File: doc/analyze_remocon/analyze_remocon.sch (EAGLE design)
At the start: 15 parts, among them IC3 PIC18F2550_28DIP, T1 2SC1815, X1 MINI-USB-UX60-MB-5S8

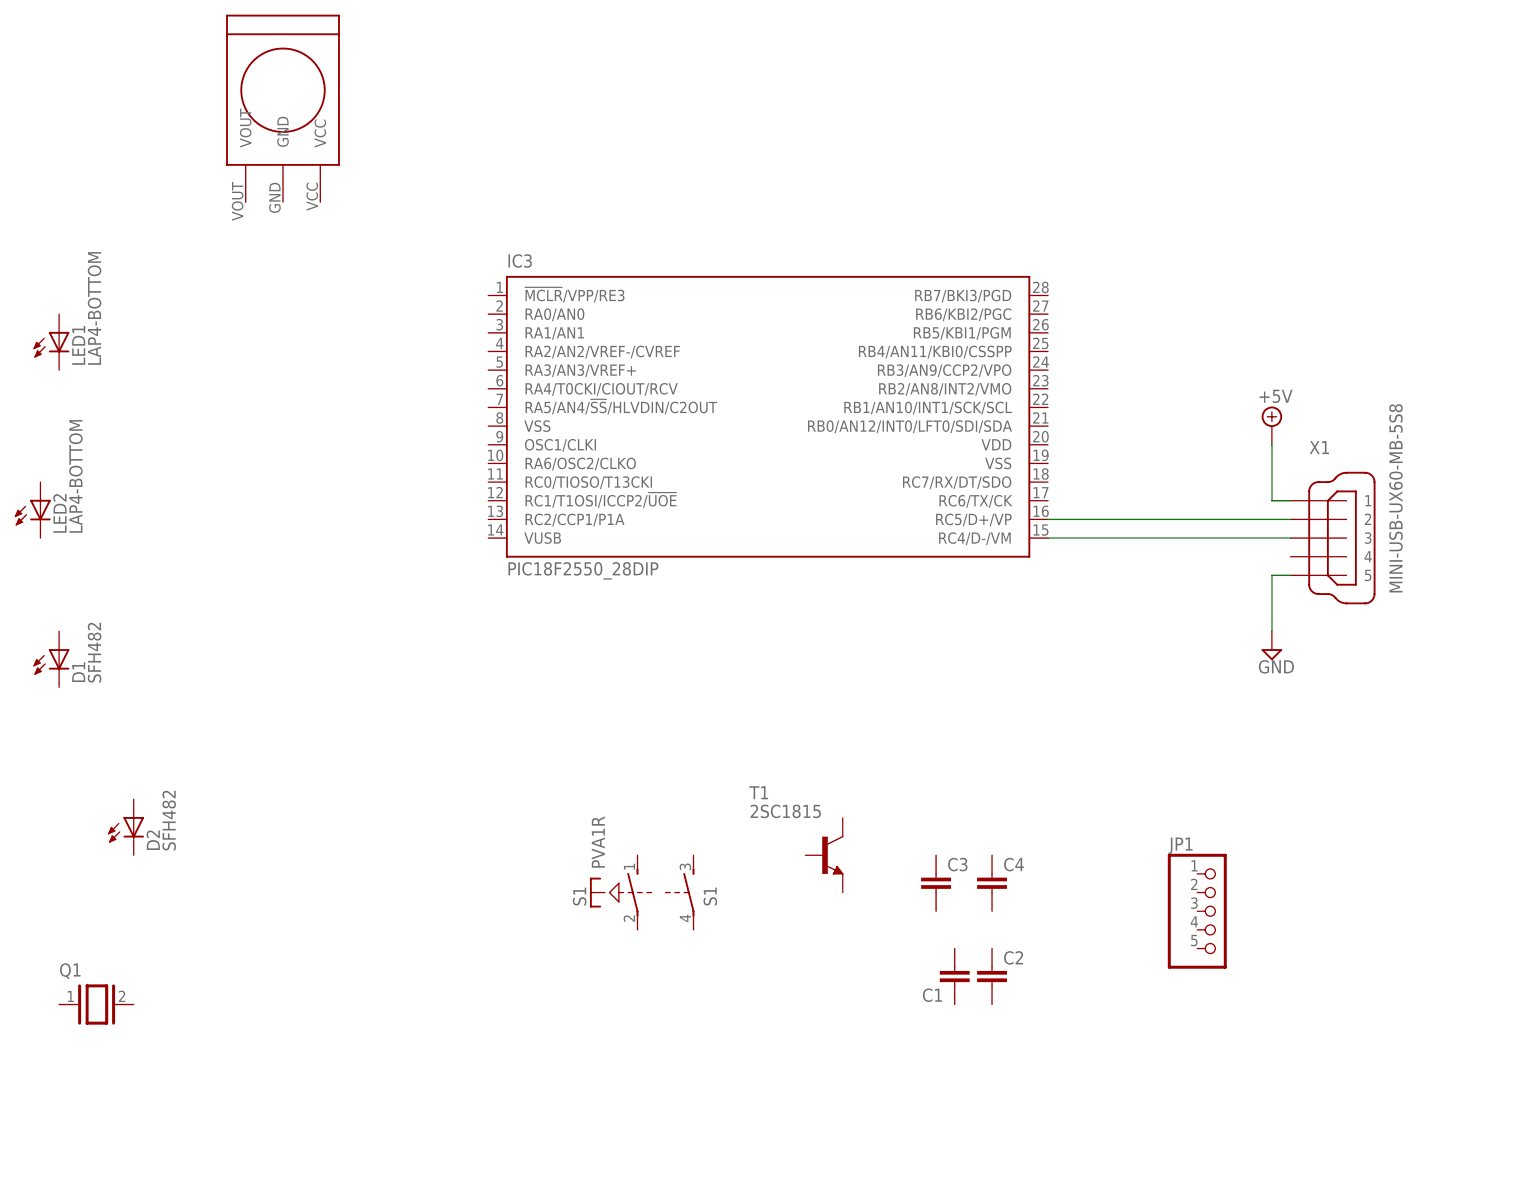
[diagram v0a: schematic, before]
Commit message: update circuit diagram documents
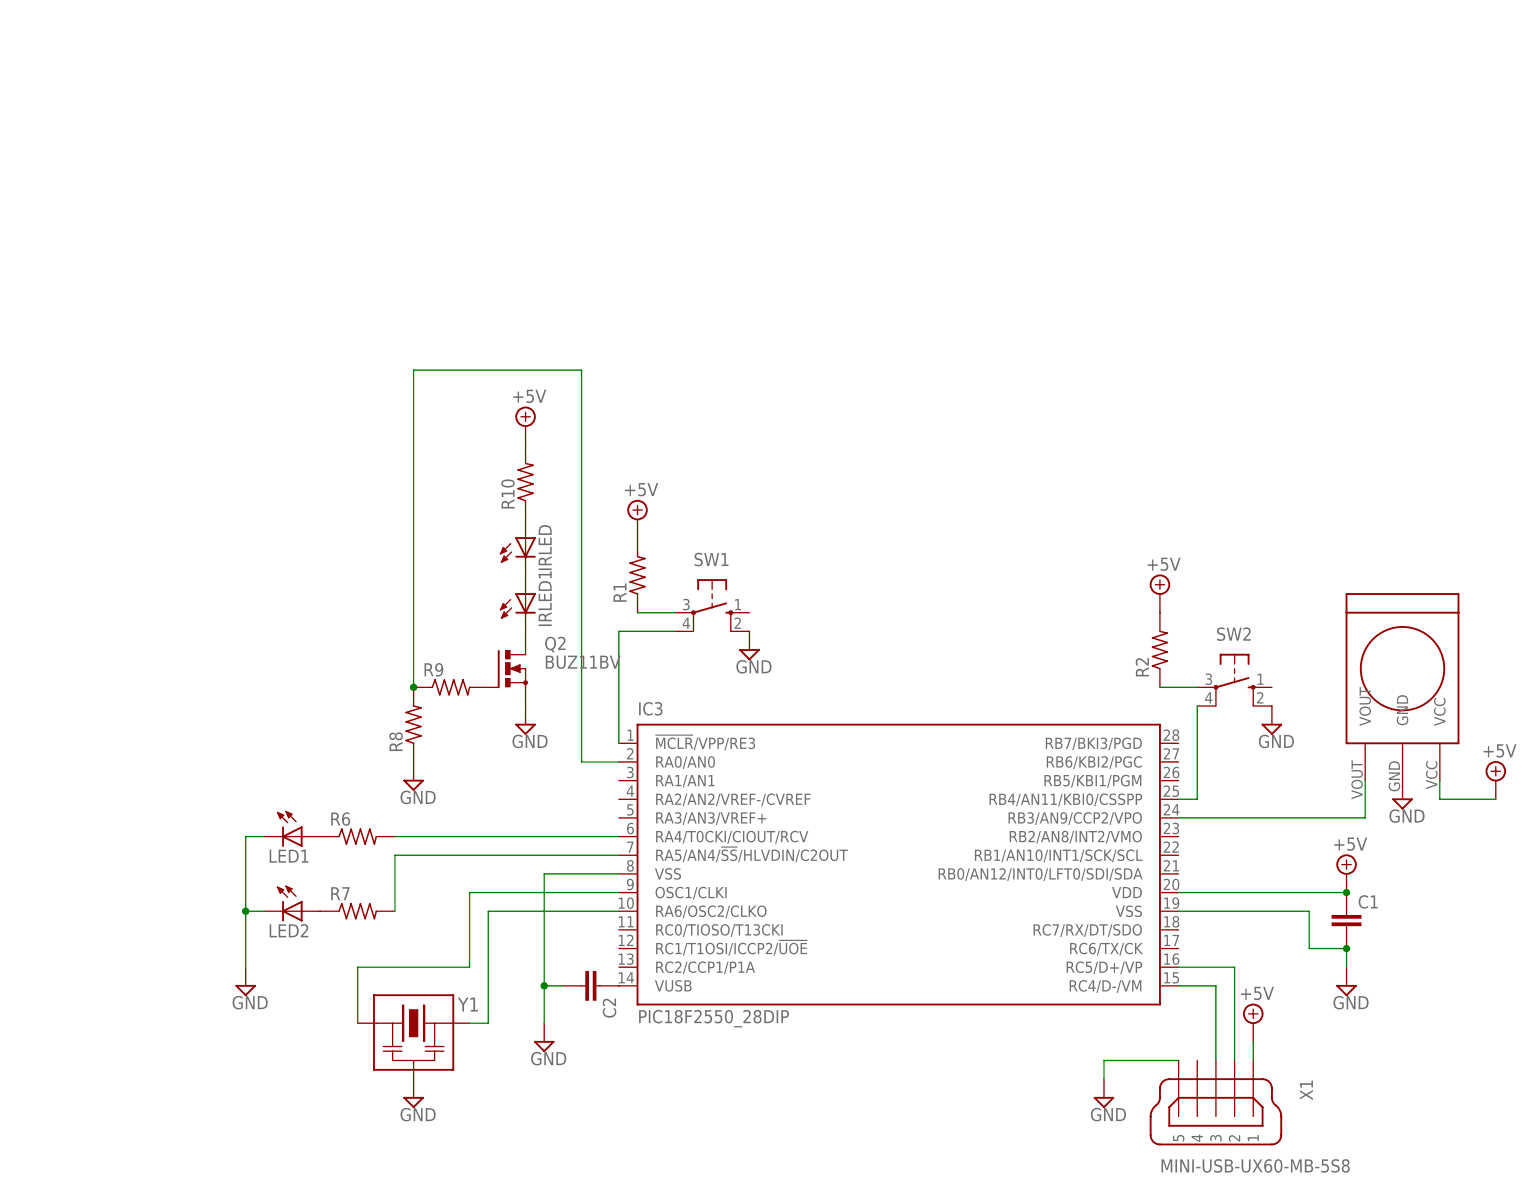
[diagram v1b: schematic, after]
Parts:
- removed C3, C4: (no value), rcl:C-EU025-024X044
- removed D1, D2: SFH482, led:SFH482
- removed JP1: (no value), pinhead:PINHD-1X5/90
- removed Q1: (no value), special:XTAL/S
- removed S1: PVA1R, switch-misc:PVA1R
- removed T1: 2SC1815, transistor:2SC1815
- added IRLED, IRLED1: (no value), led:LED3MM
- added Q2: BUZ11BV, transistor-power:BUZ11BV
- added R1, R2, R6, R7: (no value), rcl:R-US_MELF0102R
- added R10, R8, R9: (no value), rcl:R-US_0207/7
- added SW1, SW2: (no value), switch-omron:10-XX
- added Y1: (no value), xtal:CRES-HA
- C1, C2: device rcl:C-EU025-024X044 -> rcl:C-EUC0603K
- LED1, LED2: value LAP4-BOTTOM -> (none); device led:LAP4-BOTTOM -> led:LED3MM
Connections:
- removed net +5V: X1.1
- new net 20MHZ: IC3.OSC1/CLKI, Y1.LFT
- new net BLOCK: C1.1, IC3.VDD, R1.2, R10.2, R2.2, U$1.VCC, X1.1
- new net N$10: C2.1, IC3.VUSB
- new net N$11: LED1.A, R6.1
- new net N$12: IC3.RA5/AN4/!SS!/HLVDIN/C2OUT, R7.2
- new net N$13: LED2.A, R7.1
- new net N$14: IC3.RA0/AN0, R8.2, R9.1
- new net N$15: IRLED.A, R10.1
- new net N$16: IRLED.C, IRLED1.A
- new net N$17: IRLED1.C, Q2.D
- new net N$18: Q2.G, R9.2
- new net N$3: R1.1, SW1.P
- new net N$4: IC3.!MCLR!/VPP/RE3, SW1.P1
- new net N$5: R2.1, SW2.P
- new net N$6: IC3.RB4/AN11/KBI0/CSSPP, SW2.P1
- new net N$7: IC3.RB3/AN9/CCP2/VPO, U$1.VOUT
- new net N$8: IC3.RA6/OSC2/CLKO, Y1.RIT
- new net N$9: IC3.RA4/T0CKI/CIOUT/RCV, R6.2
- net GND: now also C1.2, C2.2, IC3.VSS, IC3.VSS@1, LED1.C, LED2.C, Q2.S, R8.1, SW1.S1, SW2.S1, U$1.GND, Y1.GND
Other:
- moved on the sheet: C1, C2, IC3, LED1, LED2, X1

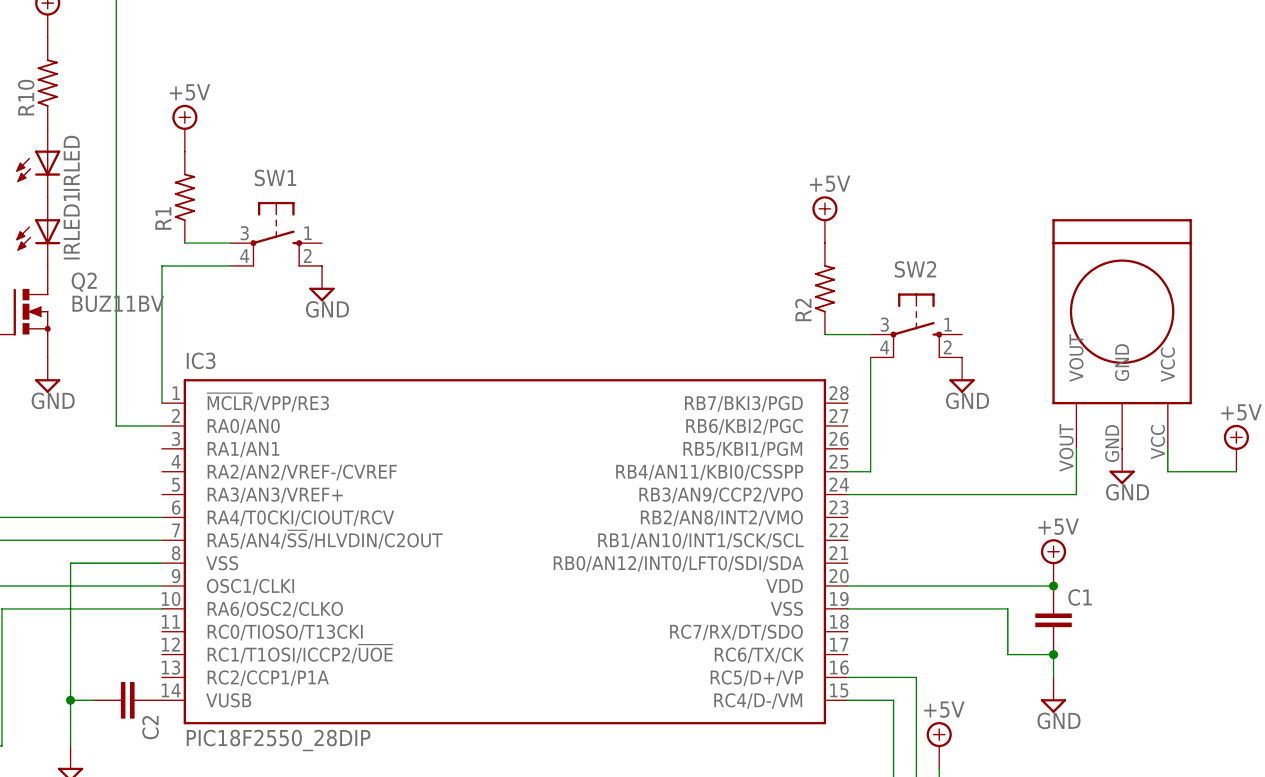
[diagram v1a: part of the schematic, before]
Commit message: update circuit diagram documents
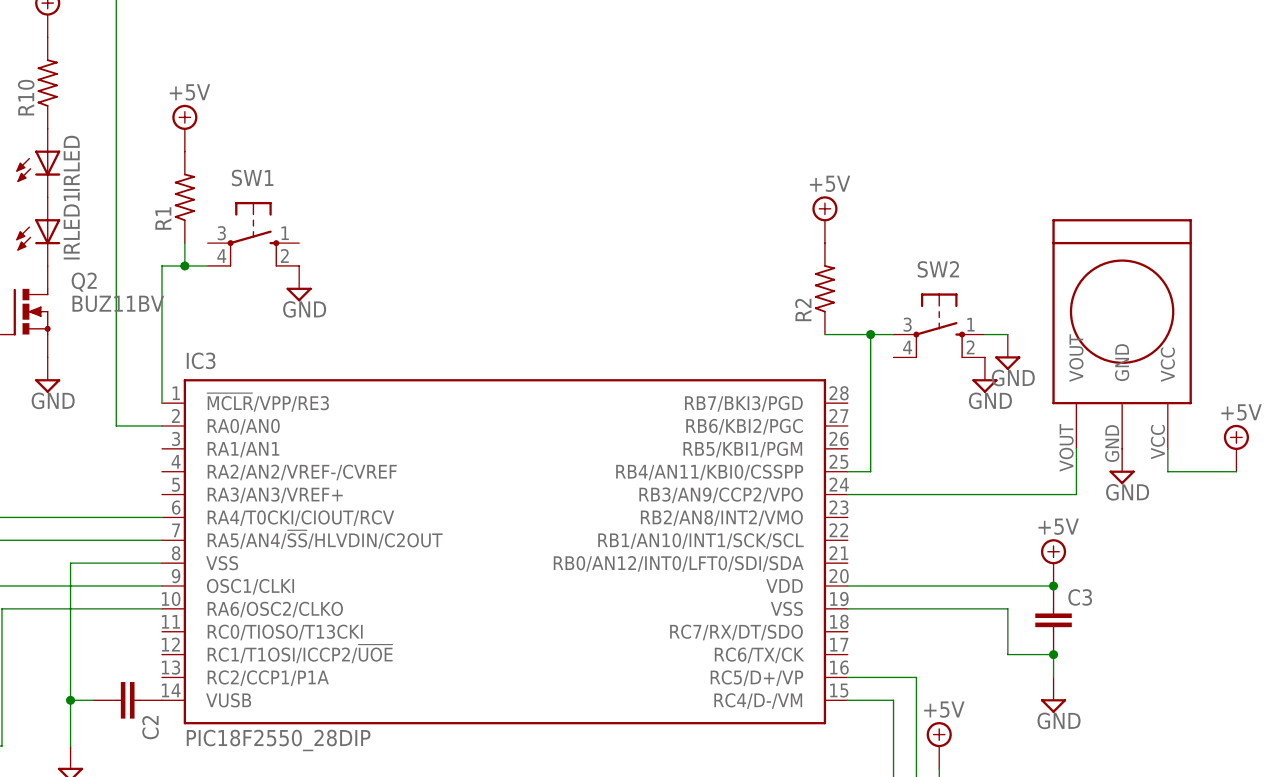
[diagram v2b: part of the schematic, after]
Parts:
- removed C1: (no value), rcl:C-EUC0603K
- added C3: (no value), rcl:C-EU025-025X050
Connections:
- removed net N$3: R1.1, SW1.P
- removed net N$5: R2.1, SW2.P
- removed net N$6: IC3.RB4/AN11/KBI0/CSSPP, SW2.P1
- new net N$7: IC3.RB4/AN11/KBI0/CSSPP, R2.1, SW2.P
- net BLOCK: now also C3.1; no longer C1.1
- net GND: now also C3.2, SW2.S; no longer C1.2
- net N$4: now also R1.1
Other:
- moved on the sheet: SW1, SW2
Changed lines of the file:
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@@
 <part name="LED2" library="led" deviceset="LED" device="3MM"/>
 <part name="Y1" library="xtal" deviceset="CRES-H" device="A"/>
-<part name="C1" library="rcl" deviceset="C-EU" device="C0603K"/>
 <part name="C2" library="rcl" deviceset="C-EU" device="C0603K"/>
 <part name="R1" library="rcl" deviceset="R-US_" device="MELF0102R"/>
@@
 <part name="R10" library="rcl" deviceset="R-US_" device="0207/7"/>
 <part name="Q2" library="transistor-power" deviceset="BUZ11" device="BV"/>
+<part name="C3" library="rcl" deviceset="C-EU" device="025-025X050"/>
+<part name="SUPPLY17" library="supply2" deviceset="GND" device=""/>
 </parts>
 <sheets>
@@
 <instance part="SUPPLY3" gate="+5V" x="96.52" y="17.78"/>
 <instance part="SUPPLY4" gate="GND" x="96.52" y="2.54"/>
-<instance part="SW1" gate="1" x="10.16" y="53.34" rot="R270"/>
-<instance part="SW2" gate="1" x="81.28" y="43.18" rot="R270"/>
+<instance part="SW1" gate="1" x="7.62" y="53.34" rot="R270"/>
+<instance part="SW2" gate="1" x="83.82" y="43.18" rot="R270"/>
 <instance part="SUPPLY5" gate="+5V" x="0" y="66.04"/>
-<instance part="SUPPLY6" gate="GND" x="15.24" y="48.26"/>
+<instance part="SUPPLY6" gate="GND" x="12.7" y="48.26"/>
 <instance part="SUPPLY7" gate="+5V" x="71.12" y="55.88"/>
 <instance part="SUPPLY8" gate="+5V" x="116.84" y="30.48"/>
 <instance part="SUPPLY9" gate="GND" x="104.14" y="27.94"/>
-<instance part="SUPPLY10" gate="GND" x="86.36" y="38.1"/>
+<instance part="SUPPLY10" gate="GND" x="88.9" y="38.1"/>
 <instance part="SUPPLY11" gate="GND" x="-12.7" y="-5.08"/>
 <instance part="SUPPLY12" gate="GND" x="-53.34" y="2.54"/>
@@
 <instance part="LED2" gate="G$1" x="-45.72" y="12.7" rot="R270"/>
 <instance part="Y1" gate="G$1" x="-30.48" y="-2.54"/>
-<instance part="C1" gate="G$1" x="96.52" y="12.7"/>
 <instance part="C2" gate="G$1" x="-5.08" y="2.54" rot="R270"/>
 <instance part="R1" gate="G$1" x="0" y="58.42" rot="R90"/>
@@
 <instance part="R10" gate="G$1" x="-15.24" y="71.12" rot="R90"/>
 <instance part="Q2" gate="1" x="-17.78" y="45.72"/>
+<instance part="C3" gate="G$1" x="96.52" y="12.7"/>
+<instance part="SUPPLY17" gate="GND" x="91.44" y="40.64"/>
 </instances>
 <busses>
@@
 <pinref part="SUPPLY3" gate="+5V" pin="+5V"/>
 <wire x1="73.66" y1="15.24" x2="96.52" y2="15.24" width="0.1524" layer="91"/>
-<pinref part="C1" gate="G$1" pin="1"/>
+<pinref part="C3" gate="G$1" pin="1"/>
 <junction x="96.52" y="15.24"/>
 </segment>
@@
 <pinref part="SUPPLY4" gate="GND" pin="GND"/>
 <wire x1="96.52" y1="7.62" x2="96.52" y2="5.08" width="0.1524" layer="91"/>
-<pinref part="C1" gate="G$1" pin="2"/>
+<pinref part="C3" gate="G$1" pin="2"/>
 <junction x="96.52" y="7.62"/>
 </segment>
@@
 <pinref part="SUPPLY15" gate="GND" pin="GND"/>
 </segment>
+<segment>
+<pinref part="SW2" gate="1" pin="S"/>
+<pinref part="SUPPLY17" gate="GND" pin="GND"/>
+<wire x1="88.9" y1="43.18" x2="91.44" y2="43.18" width="0.1524" layer="91"/>
+</segment>
 </net>
 <net name="N$1" class="0">
@@
 </segment>
 </net>
-<net name="N$5" class="0">
-<segment>
-<pinref part="SW2" gate="1" pin="P"/>
-<wire x1="71.12" y1="43.18" x2="76.2" y2="43.18" width="0.1524" layer="91"/>
-<pinref part="R2" gate="G$1" pin="1"/>
-</segment>
-</net>
-<net name="N$6" class="0">
-<segment>
-<pinref part="IC3" gate="G$1" pin="RB4/AN11/KBI0/CSSPP"/>
-<pinref part="SW2" gate="1" pin="P1"/>
-<wire x1="73.66" y1="27.94" x2="76.2" y2="27.94" width="0.1524" layer="91"/>
-<wire x1="76.2" y1="27.94" x2="76.2" y2="40.64" width="0.1524" layer="91"/>
-</segment>
-</net>
-<net name="N$7" class="0">
+<net name="N$19" class="0">
 <segment>
 <pinref part="IC3" gate="G$1" pin="RB3/AN9/CCP2/VPO"/>
@@
 <pinref part="SW1" gate="1" pin="P1"/>
 <pinref part="IC3" gate="G$1" pin="!MCLR!/VPP/RE3"/>
-<wire x1="5.08" y1="50.8" x2="-2.54" y2="50.8" width="0.1524" layer="91"/>
+<wire x1="2.54" y1="50.8" x2="0" y2="50.8" width="0.1524" layer="91"/>
+<wire x1="0" y1="50.8" x2="-2.54" y2="50.8" width="0.1524" layer="91"/>
 <wire x1="-2.54" y1="50.8" x2="-2.54" y2="35.56" width="0.1524" layer="91"/>
-</segment>
-</net>
-<net name="N$3" class="0">
-<segment>
-<pinref part="SW1" gate="1" pin="P"/>
-<wire x1="0" y1="53.34" x2="5.08" y2="53.34" width="0.1524" layer="91"/>
 <pinref part="R1" gate="G$1" pin="1"/>
+<wire x1="0" y1="50.8" x2="0" y2="53.34" width="0.1524" layer="91"/>
+<junction x="0" y="50.8"/>
 </segment>
 </net>
@@
 </segment>
 </net>
+<net name="N$7" class="0">
+<segment>
+<pinref part="SW2" gate="1" pin="P"/>
+<wire x1="71.12" y1="43.18" x2="76.2" y2="43.18" width="0.1524" layer="91"/>
+<pinref part="R2" gate="G$1" pin="1"/>
+<pinref part="IC3" gate="G$1" pin="RB4/AN11/KBI0/CSSPP"/>
+<wire x1="76.2" y1="43.18" x2="78.74" y2="43.18" width="0.1524" layer="91"/>
+<wire x1="73.66" y1="27.94" x2="76.2" y2="27.94" width="0.1524" layer="91"/>
+<wire x1="76.2" y1="27.94" x2="76.2" y2="43.18" width="0.1524" layer="91"/>
+<junction x="76.2" y="43.18"/>
+</segment>
+</net>
